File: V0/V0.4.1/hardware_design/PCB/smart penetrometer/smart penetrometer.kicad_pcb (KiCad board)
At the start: 4 copper layers, 29 x 83.8 mm, 26 parts, among them J1 Conn_01x02_Female, J2 XLR3_Switched, J3 Conn_01x07_Female, J4 Screw_Terminal, U1 ADS1120-PW, U2 DS3231M, U3 4023, U4 ADS1115IDGS, U5 VO615A

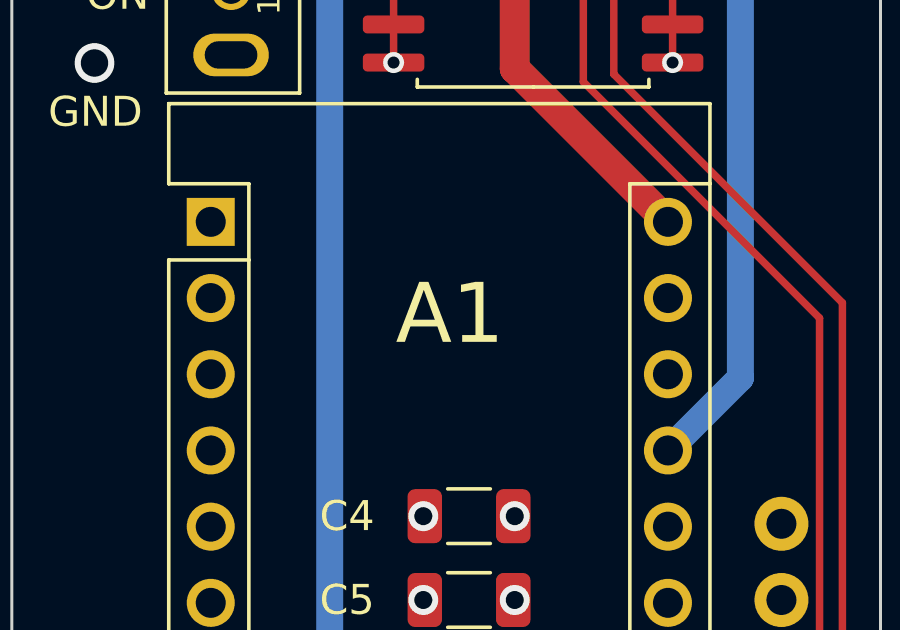
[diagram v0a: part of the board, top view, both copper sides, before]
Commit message: PCB UPDATE
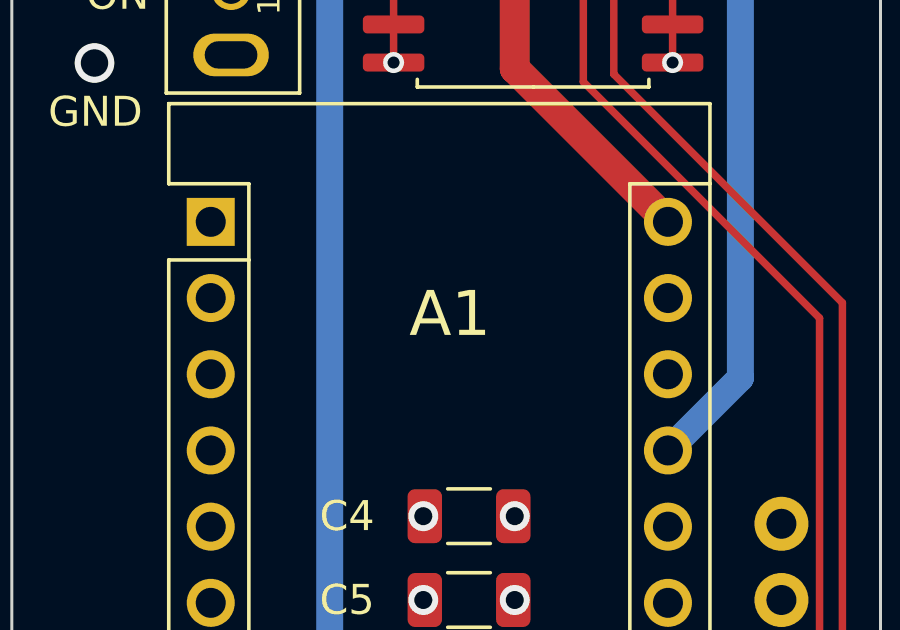
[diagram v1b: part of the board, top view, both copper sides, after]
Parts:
- added G***: LOGO, kitest:ARTS_lab_logo, B.Cu at (180.5, 86.9)
- moved G*** 1.00 mm to (180.5, 76.7)
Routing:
- added copper zone on In2.Cu, net 3V3
- added copper zone on In1.Cu, net GND
- removed copper zone on In1.Cu, net 3V3
- removed copper zone on In2.Cu, net GND
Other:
- board text added: "OPTOCOUPLER"
- board text added: "TERMINALS"
